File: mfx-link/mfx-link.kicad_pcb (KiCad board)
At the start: 2 copper layers, 50 x 50 mm, 55 parts, among them P1 CONN_01X02, P2 CONN_02X03, P3 CONN_01X02, P4 Grove I2C, P5 IBT-2, P6 CONN_01X02, P7 CONN_01X03, Q1 BC547, Q2 BC547, Q3 BC547, Q4 BC547, U1 LM393-1, U2 7805, U3 PIC16F1705, U4 6N137, U5 7805

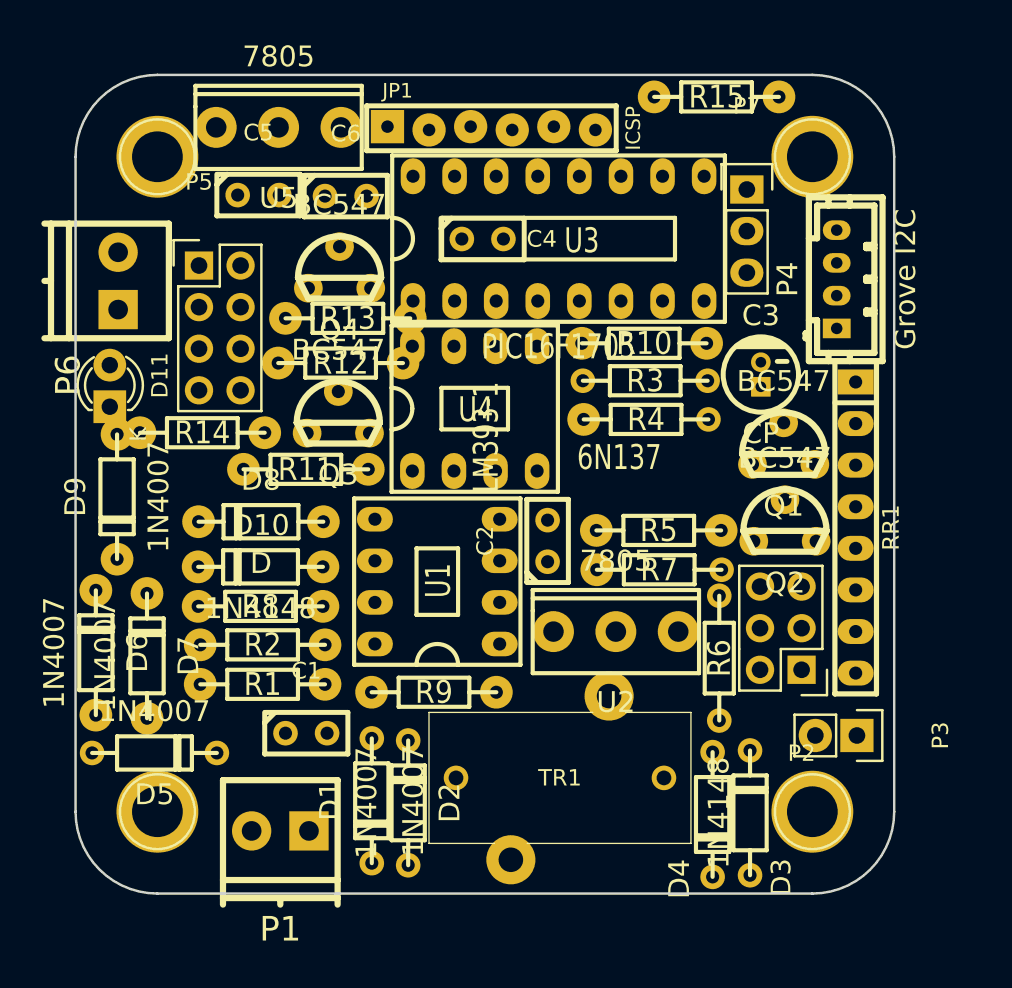
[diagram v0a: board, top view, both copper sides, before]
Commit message: wip
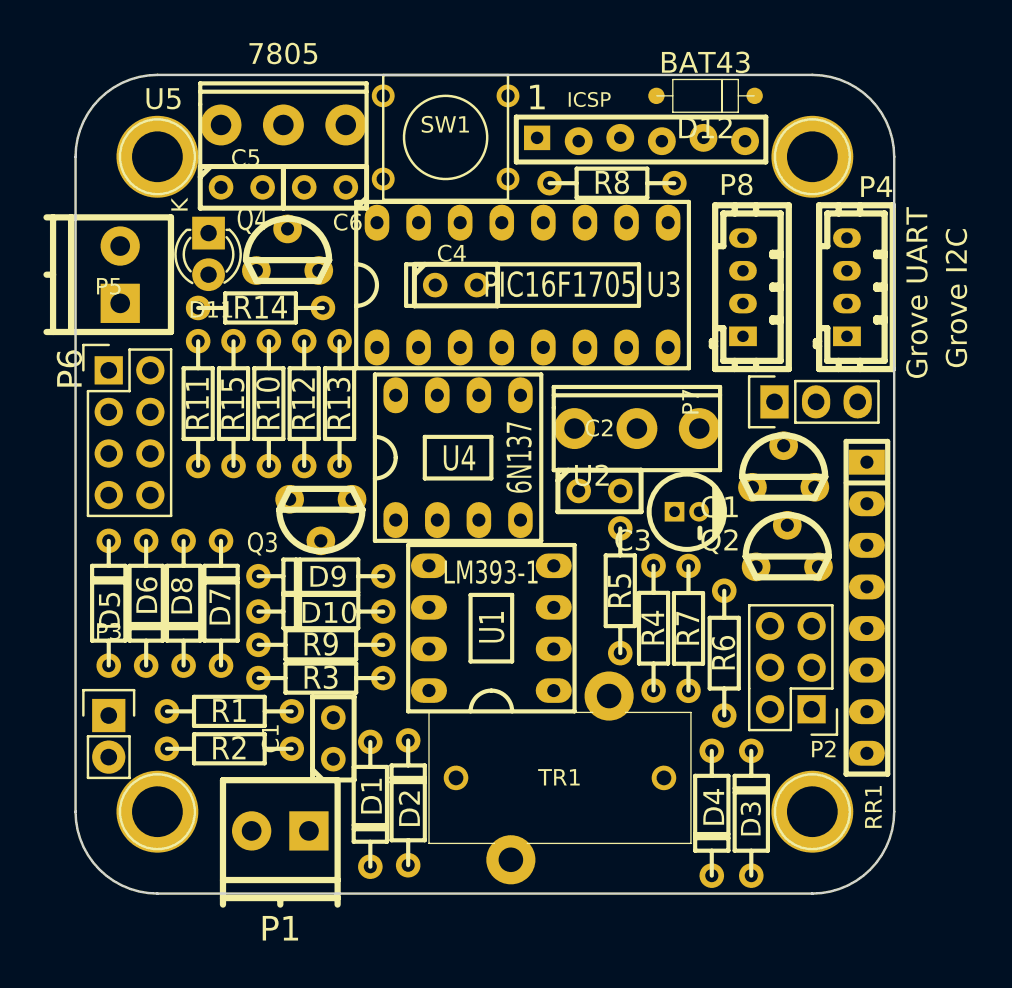
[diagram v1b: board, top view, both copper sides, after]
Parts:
- added D12: BAT43, w_pth_diodes:diode_do35, F.Cu at (133.5, 81.3)
- added P8: Grove UART, w_conn_jst-ph:b4b-ph-kl, F.Cu at (135.8, 93.0)
- added SW1: SW_PUSH, Buttons_Switches_ThroughHole:SW_PUSH_SMALL, F.Cu at (117.6, 83.8)
- moved P3 45.7 mm to (97.0, 119.1), turned to 0 degrees
- moved R15 34.9 mm to (104.6, 100.1), turned to 270 degrees
- moved R8 33.6 mm to (127.8, 86.6), turned to 0 degrees
- moved R3 26.9 mm to (110.0, 116.8), turned to 180 degrees
- moved R10 23.2 mm to (106.8, 100.1), turned to 270 degrees
- moved D9 13.4 mm to (110.0, 110.6), turned to 180 degrees
- moved P7 13.1 mm to (137.7, 100.0), turned to 90 degrees
- moved R4 12.8 mm to (130.3, 113.8), turned to 270 degrees
- moved U2 12.5 mm to (129.3, 101.6)
- moved D11 12.2 mm to (103.1, 89.7), turned to 270 degrees
- moved D5 9.56 mm to (97.0, 112.3), turned to 90 degrees
- moved C3 9.52 mm to (132.3, 106.7), turned to 270 degrees
- moved JP1 9.16 mm to (123.2, 83.9)
- moved P5 8.45 mm to (97.0, 98.0)
- moved R14 8.41 mm to (106.3, 94.2)
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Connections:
- R8 pad 2: VDD -> Net-(D12-Pad1)
- U3 pad 8: Net-(U3-Pad8) -> /TxD
- U3 pad 9: Net-(U3-Pad9) -> /RxD
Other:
- board text added: "1"

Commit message: wip
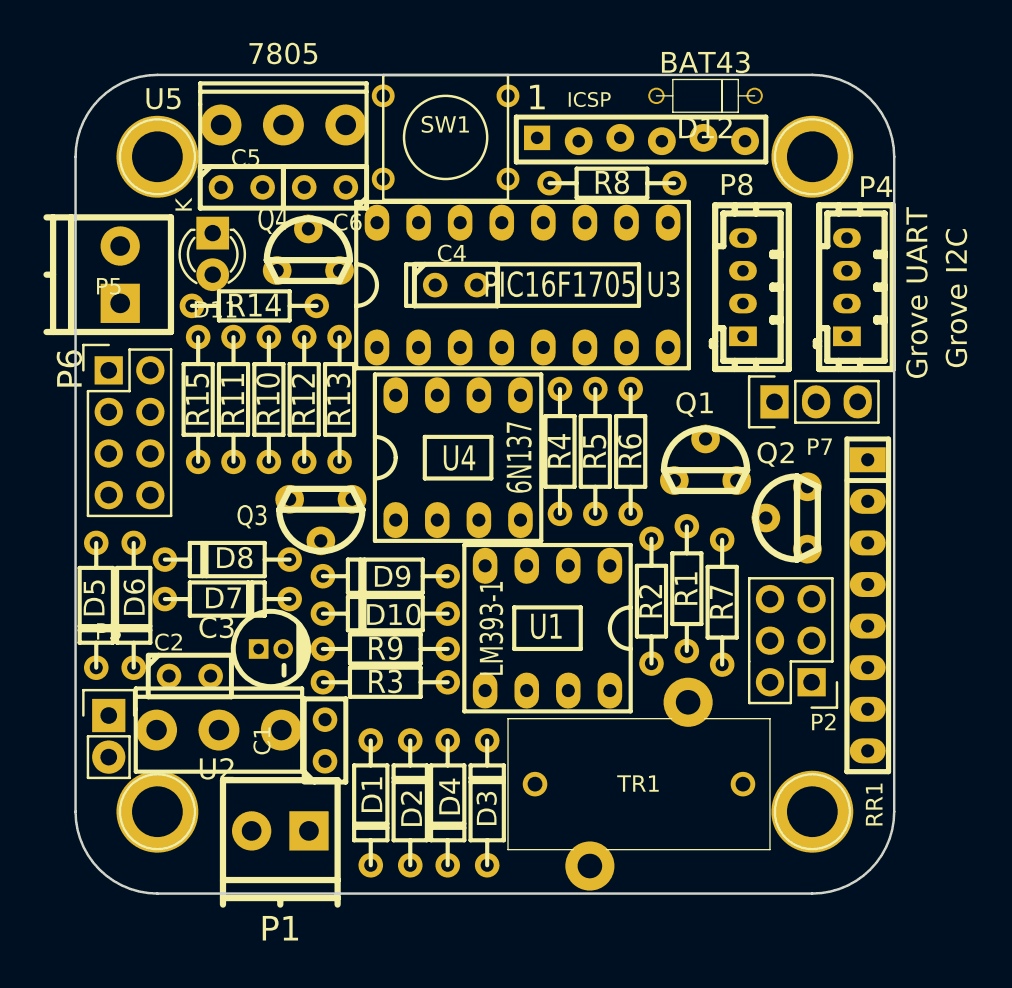
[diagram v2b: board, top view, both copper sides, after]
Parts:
- moved U2 31.5 mm to (103.8, 120.0)
- moved R1 28.9 mm to (132.3, 111.4), turned to 270 degrees
- moved C2 27.5 mm to (102.0, 116.7)
- moved R2 27.3 mm to (130.2, 112.1), turned to 270 degrees
- moved C3 26.7 mm to (106.9, 115.1)
- moved D4 16.1 mm to (117.7, 124.5)
- moved D3 16.1 mm to (120.1, 124.5)
- moved R6 13.6 mm to (128.9, 103.0)
- moved R4 12.2 mm to (124.6, 103.0)
- moved R5 8.64 mm to (126.7, 103.0), turned to 270 degrees
- moved TR1 4.84 mm to (129.4, 123.3)
- moved Q1 4.79 mm to (133.5, 104.1)
- moved R3 3.95 mm to (113.9, 117.1)
- moved R9 3.95 mm to (113.9, 115.1)
- moved D10 3.94 mm to (113.9, 112.9)
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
